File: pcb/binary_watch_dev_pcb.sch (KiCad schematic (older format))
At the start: 67 parts, among them K1 PWR_SELECT, M1 MNT, M2 MNT, M3 MNT, M4 MNT, P1 ISP, P2 USB-MICRO-B, P3 LED_ISENSE, P7 MCU_ISENSE, P8 TST, P9 TST, SW1A1 BUTTON_1, SW1B1 BUTTON_1, SW2A1 BUTTON_2, SW2B1 BUTTON_2, SW3 RESET, U1 ATMEGA168PA-A, U2 INA210, U3 NCP1117ST33T3G, U4 INA213, X1 32.768kHz

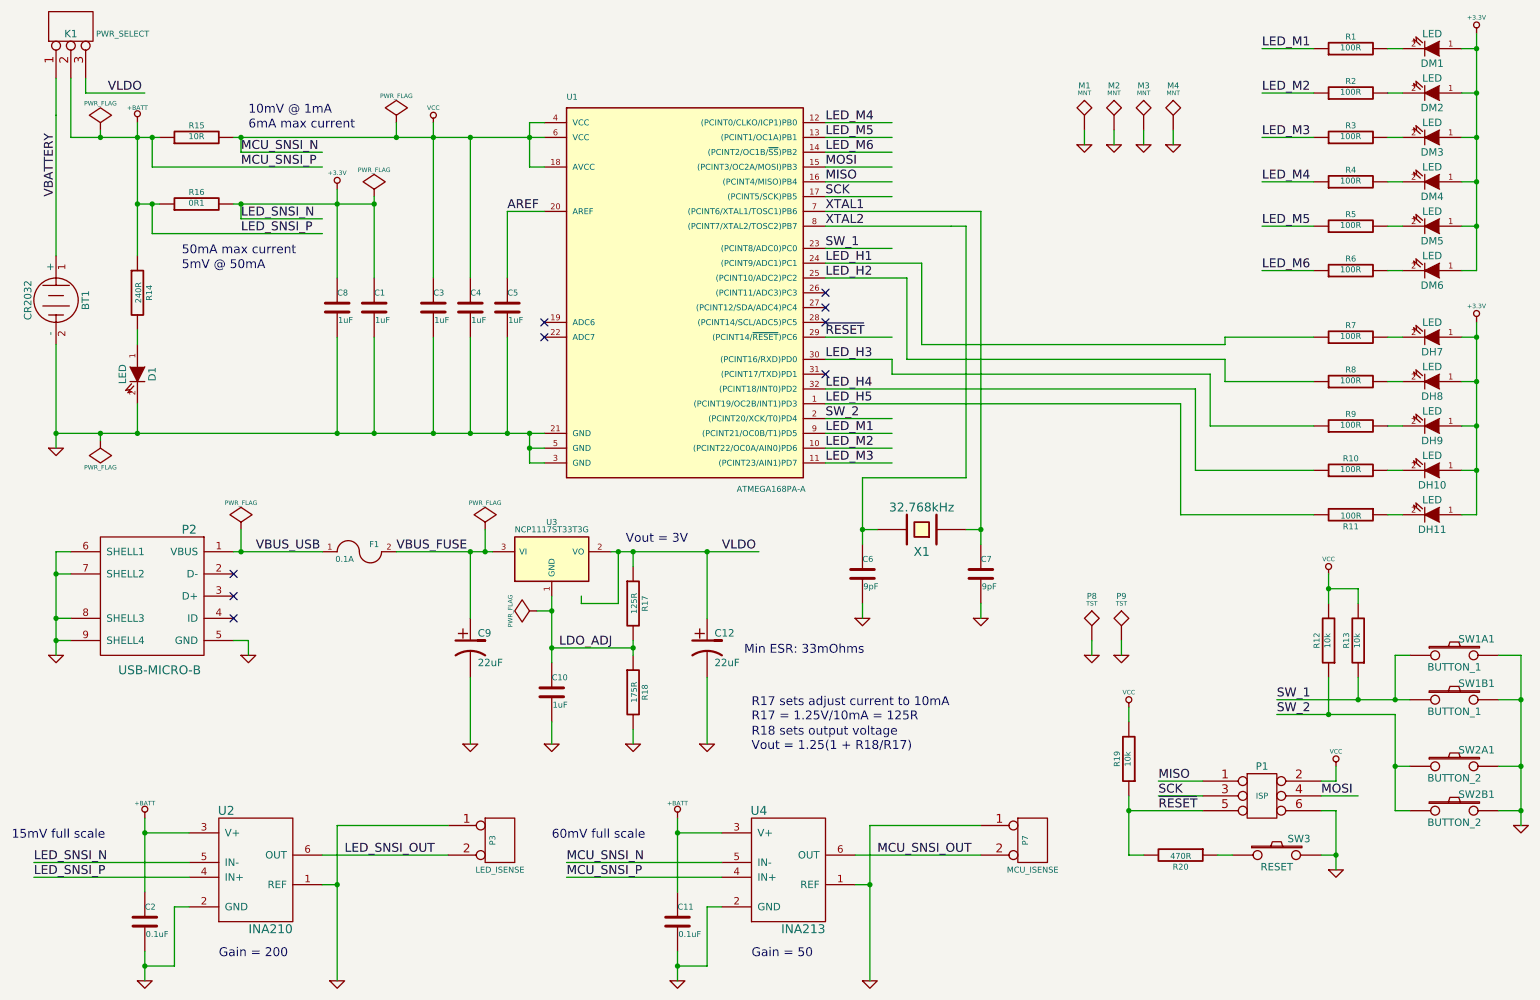
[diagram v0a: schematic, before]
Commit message: Add new dev pcb files from nightly build of kicad
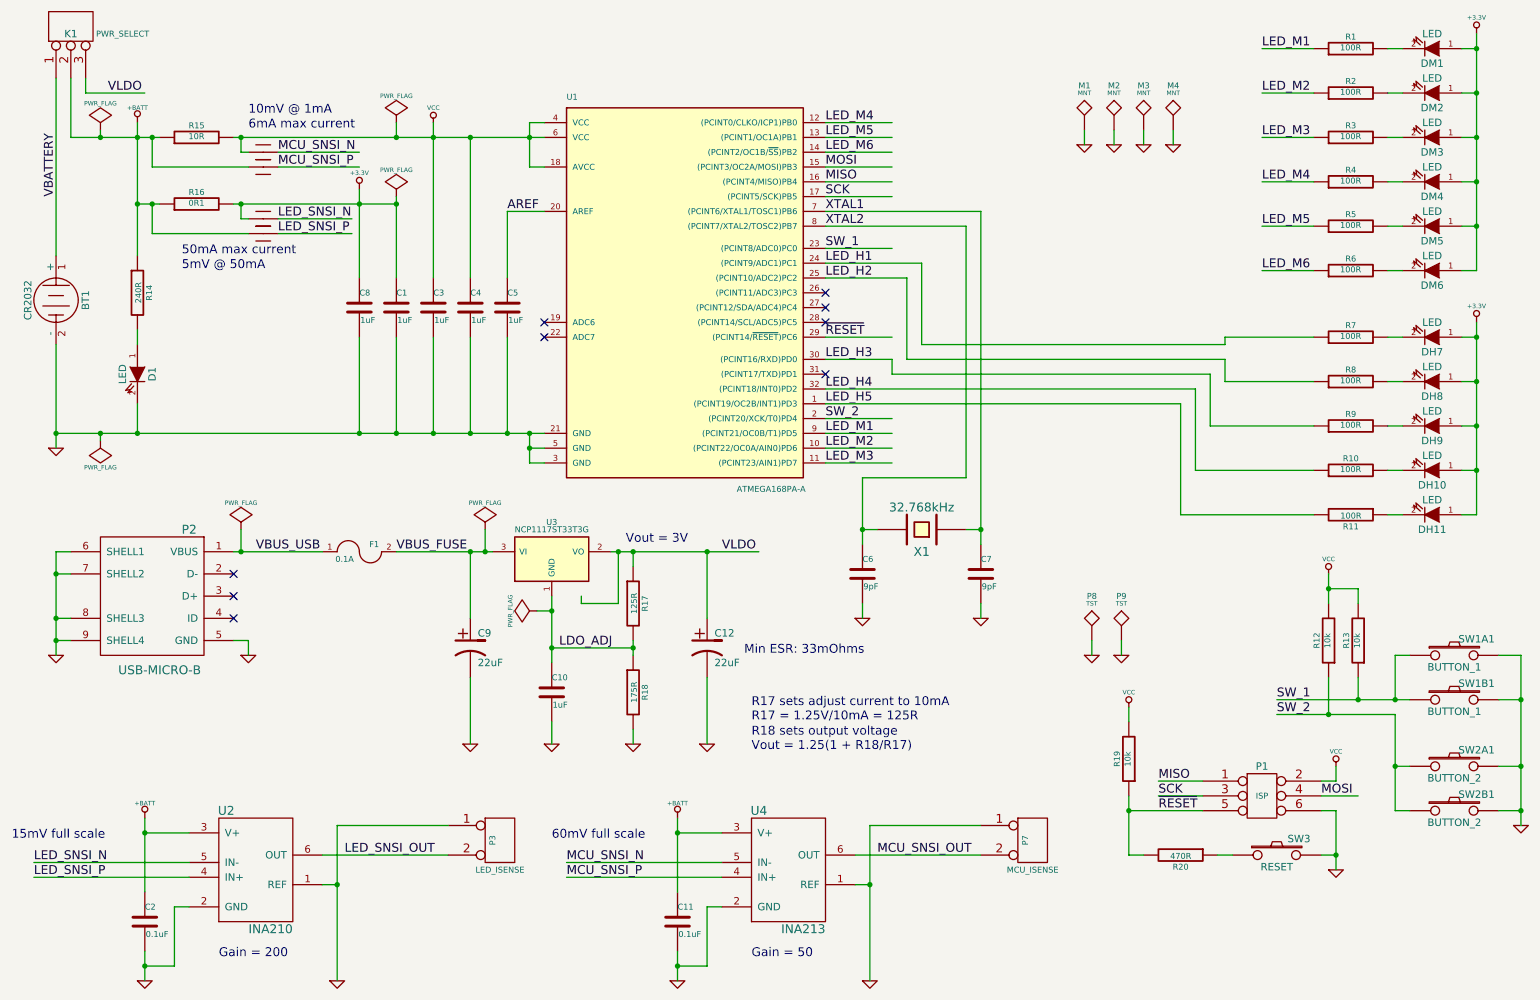
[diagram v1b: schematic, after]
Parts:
- added NET? (x4): NET_CONN, symbol NET_CONN
- C6, C7: footprint Capacitors_SMD:C_0603_HandSoldering -> Capacitors_SMD:C_0402
- SW1A1, SW2A1: Manufacturer P/N (none) -> EVQ-P7C01P; Vendor P/N (none) -> P16765CT-ND
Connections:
- wire segments 269 -> 204
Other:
- moved on the sheet: C1, C8
